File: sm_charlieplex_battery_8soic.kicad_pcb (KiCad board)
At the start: 2 copper layers, 12 x 12 mm, 14 parts, among them SW1 SW_Push, U1 ATtiny402-SS

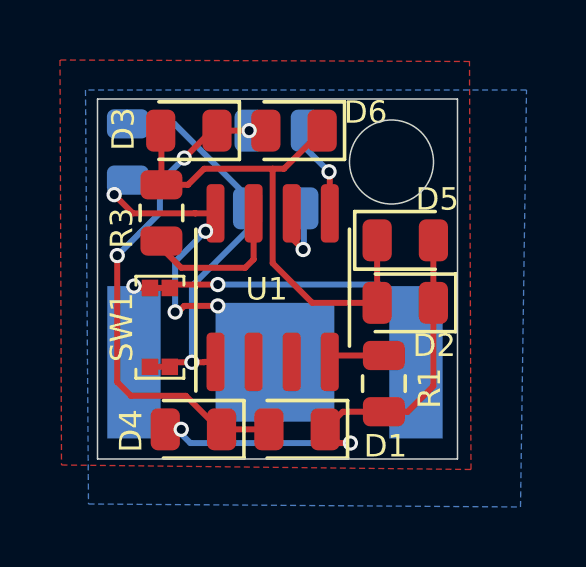
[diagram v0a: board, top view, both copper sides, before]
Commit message: Some changes
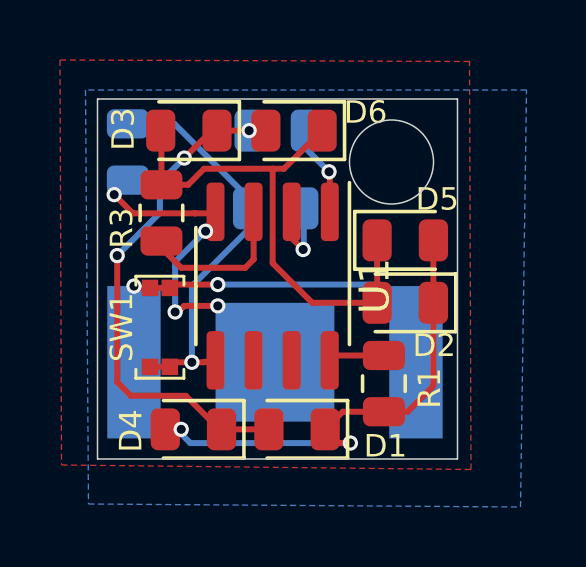
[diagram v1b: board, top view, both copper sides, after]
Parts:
- U1: value ATtiny402-SS -> ATtiny13A-SSU
- moved U1 0.05 mm to (170.7, 110.2), turned to 270 degrees
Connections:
- U1 pad 1: Net-(C1-Pad1) -> Net-(R4-Pad2)
- U1 pad 2: Net-(U1-Pad2) -> Net-(R3-Pad2)
- U1 pad 4: Net-(R1-Pad2) -> /GND
- U1 pad 5: Net-(R2-Pad2) -> Net-(U1-Pad5)
- U1 pad 6: Net-(R4-Pad2) -> Net-(R1-Pad2)
- U1 pad 7: Net-(R3-Pad2) -> Net-(R2-Pad2)
- U1 pad 8: /GND -> Net-(C1-Pad1)
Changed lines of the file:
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@@
   )
   (setup
-    (last_trace_width 0.2)
+    (last_trace_width 0.25)
     (user_trace_width 0.2)
     (trace_clearance 0.2)
@@
   (net 10 "Net-(C1-Pad1)")
   (net 11 "Net-(U1-Pad3)")
-  (net 12 "Net-(U1-Pad2)")
+  (net 12 "Net-(U1-Pad5)")
   (net_class Default "This is the default net class."
     (clearance 0.2)
@@
     (add_net "Net-(R3-Pad2)")
     (add_net "Net-(R4-Pad2)")
-    (add_net "Net-(U1-Pad2)")
     (add_net "Net-(U1-Pad3)")
+    (add_net "Net-(U1-Pad5)")
+  )
+  (module Package_SO:SOIC-8_3.9x4.9mm_P1.27mm (layer F.Cu)
+    (at 170.7388 110.236 270)
+    (descr "SOIC, 8 Pin (JEDEC MS-012AA, https://www.analog.com/media/en/package-pcb-resources/package/pkg_pdf/soic_narrow-r/r_8.pdf), generated with kicad-footprint-generator ipc_gullwing_generator.py")
+    (tags "SOIC SO")
+    (attr smd)
+    (fp_text reference U1 (at 0 -3.4 90) (layer F.SilkS)
+      (effects (font (size 1 1) (thickness 0.15)))
+    )
+    (fp_text value ATtiny13A-SSU (at 0 3.4 90) (layer F.Fab)
+      (effects (font (size 1 1) (thickness 0.15)))
+    )
+    (fp_text user %R (at 0 0 90) (layer F.Fab)
+      (effects (font (size 0.98 0.98) (thickness 0.15)))
+    )
+    (fp_line (start 3.7 -2.7) (end -3.7 -2.7) (layer F.CrtYd) (width 0.05))
+    (fp_line (start 3.7 2.7) (end 3.7 -2.7) (layer F.CrtYd) (width 0.05))
+    (fp_line (start -3.7 2.7) (end 3.7 2.7) (layer F.CrtYd) (width 0.05))
+    (fp_line (start -3.7 -2.7) (end -3.7 2.7) (layer F.CrtYd) (width 0.05))
+    (fp_line (start -1.95 -1.475) (end -0.975 -2.45) (layer F.Fab) (width 0.1))
+    (fp_line (start -1.95 2.45) (end -1.95 -1.475) (layer F.Fab) (width 0.1))
+    (fp_line (start 1.95 2.45) (end -1.95 2.45) (layer F.Fab) (width 0.1))
+    (fp_line (start 1.95 -2.45) (end 1.95 2.45) (layer F.Fab) (width 0.1))
+    (fp_line (start -0.975 -2.45) (end 1.95 -2.45) (layer F.Fab) (width 0.1))
+    (fp_line (start 0 -2.56) (end -3.45 -2.56) (layer F.SilkS) (width 0.12))
+    (fp_line (start 0 -2.56) (end 1.95 -2.56) (layer F.SilkS) (width 0.12))
+    (fp_line (start 0 2.56) (end -1.95 2.56) (layer F.SilkS) (width 0.12))
+    (fp_line (start 0 2.56) (end 1.95 2.56) (layer F.SilkS) (width 0.12))
+    (pad 8 smd roundrect (at 2.475 -1.905 270) (size 1.95 0.6) (layers F.Cu F.Paste F.Mask) (roundrect_rratio 0.25)
+      (net 10 "Net-(C1-Pad1)"))
+    (pad 7 smd roundrect (at 2.475 -0.635 270) (size 1.95 0.6) (layers F.Cu F.Paste F.Mask) (roundrect_rratio 0.25)
+      (net 6 "Net-(R2-Pad2)"))
+    (pad 6 smd roundrect (at 2.475 0.635 270) (size 1.95 0.6) (layers F.Cu F.Paste F.Mask) (roundrect_rratio 0.25)
+      (net 5 "Net-(R1-Pad2)"))
+    (pad 5 smd roundrect (at 2.475 1.905 270) (size 1.95 0.6) (layers F.Cu F.Paste F.Mask) (roundrect_rratio 0.25)
+      (net 12 "Net-(U1-Pad5)"))
+    (pad 4 smd roundrect (at -2.475 1.905 270) (size 1.95 0.6) (layers F.Cu F.Paste F.Mask) (roundrect_rratio 0.25)
+      (net 4 /GND))
+    (pad 3 smd roundrect (at -2.475 0.635 270) (size 1.95 0.6) (layers F.Cu F.Paste F.Mask) (roundrect_rratio 0.25)
+      (net 11 "Net-(U1-Pad3)"))
+    (pad 2 smd roundrect (at -2.475 -0.635 270) (size 1.95 0.6) (layers F.Cu F.Paste F.Mask) (roundrect_rratio 0.25)
+      (net 7 "Net-(R3-Pad2)"))
+    (pad 1 smd roundrect (at -2.475 -1.905 270) (size 1.95 0.6) (layers F.Cu F.Paste F.Mask) (roundrect_rratio 0.25)
+      (net 8 "Net-(R4-Pad2)"))
+    (model ${KISYS3DMOD}/Package_SO.3dshapes/SOIC-8_3.9x4.9mm_P1.27mm.wrl
+      (at (xyz 0 0 0))
+      (scale (xyz 1 1 1))
+      (rotate (xyz 0 0 0))
+    )
   )
   (module Battery:BatteryHolder_Keystone_2998_621_6.8x2.2mm (layer B.Cu)
@@
     (pad 2 smd rect (at 0 0) (size 3.96 3.96) (layers B.Cu B.Paste B.Mask)
       (net 4 /GND))
-  )
-  (module Package_SO:SOIC-8_3.9x4.9mm_P1.27mm (layer F.Cu)
-    (at 170.7388 110.2868 90)
-    (descr "SOIC, 8 Pin (JEDEC MS-012AA, https://www.analog.com/media/en/package-pcb-resources/package/pkg_pdf/soic_narrow-r/r_8.pdf), generated with kicad-footprint-generator ipc_gullwing_generator.py")
-    (tags "SOIC SO")
-    (attr smd)
-    (fp_text reference U1 (at -0.0508 -0.2032 180) (layer F.SilkS)
-      (effects (font (size 0.75 0.75) (thickness 0.1)))
-    )
-    (fp_text value ATtiny402-SS (at 0 3.4 90) (layer F.Fab)
-      (effects (font (size 1 1) (thickness 0.15)))
-    )
-    (fp_line (start 0 2.56) (end 1.95 2.56) (layer F.SilkS) (width 0.12))
-    (fp_line (start 0 2.56) (end -1.95 2.56) (layer F.SilkS) (width 0.12))
-    (fp_line (start 0 -2.56) (end 1.95 -2.56) (layer F.SilkS) (width 0.12))
-    (fp_line (start 0 -2.56) (end -3.45 -2.56) (layer F.SilkS) (width 0.12))
-    (fp_line (start -0.975 -2.45) (end 1.95 -2.45) (layer F.Fab) (width 0.1))
-    (fp_line (start 1.95 -2.45) (end 1.95 2.45) (layer F.Fab) (width 0.1))
-    (fp_line (start 1.95 2.45) (end -1.95 2.45) (layer F.Fab) (width 0.1))
-    (fp_line (start -1.95 2.45) (end -1.95 -1.475) (layer F.Fab) (width 0.1))
-    (fp_line (start -1.95 -1.475) (end -0.975 -2.45) (layer F.Fab) (width 0.1))
-    (fp_line (start -3.7 -2.7) (end -3.7 2.7) (layer F.CrtYd) (width 0.05))
-    (fp_line (start -3.7 2.7) (end 3.7 2.7) (layer F.CrtYd) (width 0.05))
-    (fp_line (start 3.7 2.7) (end 3.7 -2.7) (layer F.CrtYd) (width 0.05))
-    (fp_line (start 3.7 -2.7) (end -3.7 -2.7) (layer F.CrtYd) (width 0.05))
-    (fp_text user %R (at 0 0 90) (layer F.Fab)
-      (effects (font (size 0.98 0.98) (thickness 0.15)))
-    )
-    (pad 1 smd roundrect (at -2.475 -1.905 90) (size 1.95 0.6) (layers F.Cu F.Paste F.Mask) (roundrect_rratio 0.25)
-      (net 10 "Net-(C1-Pad1)"))
-    (pad 2 smd roundrect (at -2.475 -0.635 90) (size 1.95 0.6) (layers F.Cu F.Paste F.Mask) (roundrect_rratio 0.25)
-      (net 12 "Net-(U1-Pad2)"))
-    (pad 3 smd roundrect (at -2.475 0.635 90) (size 1.95 0.6) (layers F.Cu F.Paste F.Mask) (roundrect_rratio 0.25)
-      (net 11 "Net-(U1-Pad3)"))
-    (pad 4 smd roundrect (at -2.475 1.905 90) (size 1.95 0.6) (layers F.Cu F.Paste F.Mask) (roundrect_rratio 0.25)
-      (net 5 "Net-(R1-Pad2)"))
-    (pad 5 smd roundrect (at 2.475 1.905 90) (size 1.95 0.6) (layers F.Cu F.Paste F.Mask) (roundrect_rratio 0.25)
-      (net 6 "Net-(R2-Pad2)"))
-    (pad 6 smd roundrect (at 2.475 0.635 90) (size 1.95 0.6) (layers F.Cu F.Paste F.Mask) (roundrect_rratio 0.25)
-      (net 8 "Net-(R4-Pad2)"))
-    (pad 7 smd roundrect (at 2.475 -0.635 90) (size 1.95 0.6) (layers F.Cu F.Paste F.Mask) (roundrect_rratio 0.25)
-      (net 7 "Net-(R3-Pad2)"))
-    (pad 8 smd roundrect (at 2.475 -1.905 90) (size 1.95 0.6) (layers F.Cu F.Paste F.Mask) (roundrect_rratio 0.25)
-      (net 4 /GND))
-    (model ${KISYS3DMOD}/Package_SO.3dshapes/SOIC-8_3.9x4.9mm_P1.27mm.wrl
-      (at (xyz 0 0 0))
-      (scale (xyz 1 1 1))
-      (rotate (xyz 0 0 0))
-    )
   )
   (module Button_Switch_SMD:SW_Push_2.6x1.6x0.53mm_EVP-BB2A9B000 (layer F.Cu)
@@
   (gr_line (start 176.9 104) (end 176.9 116) (layer Edge.Cuts) (width 0.05))
   (gr_line (start 164.9 104) (end 176.9 104) (layer Edge.Cuts) (width 0.05))
-  (via (at 168.91 110.8964) (size 0.51) (drill 0.3) (layers F.Cu B.Cu) (net 4))
   (segment (start 173.0756 114.4247) (end 172.4891 115.0112) (width 0.2) (layer F.Cu) (net 1))
   (segment (start 174.4472 114.4247) (end 173.0756 114.4247) (width 0.2) (layer F.Cu) (net 1))
@@
   (segment (start 168.4528 106.3244) (end 170.7388 106.3244) (width 0.2) (layer F.Cu) (net 3))
   (segment (start 170.7388 106.3244) (end 171.1175 106.3244) (width 0.2) (layer F.Cu) (net 3))
+  (via (at 168.91 110.8964) (size 0.51) (drill 0.3) (layers F.Cu B.Cu) (net 4))
   (segment (start 168.8338 107.8118) (end 168.1622 107.8118) (width 0.2) (layer F.Cu) (net 4))
   (segment (start 168.1622 107.8118) (end 168.148 107.7976) (width 0.2) (layer F.Cu) (net 4))
